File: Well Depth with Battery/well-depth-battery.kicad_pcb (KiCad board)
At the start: 2 copper layers, 40.8 x 48.3 mm, 60 parts, among them J1 Conn_01x02_Female, J2 Conn_01x04_Female, J3 Micro_SD_Card, J4 Conn_01x02_Male, J5 USB_A, J6 Conn_02x05_Odd_Even, Q1 Q_NMOS_GSD, Q2 Q_PMOS_GSD, Q3 Q_PMOS_GSD, U1 LM358, U2 LM358, U3 TL431DBZ, U4 NCP1117-5.0_SOT223, U5 ATSAMD21E17D-M, U6 MCP1793T-3302H/DC, Y1 Crystal_Small

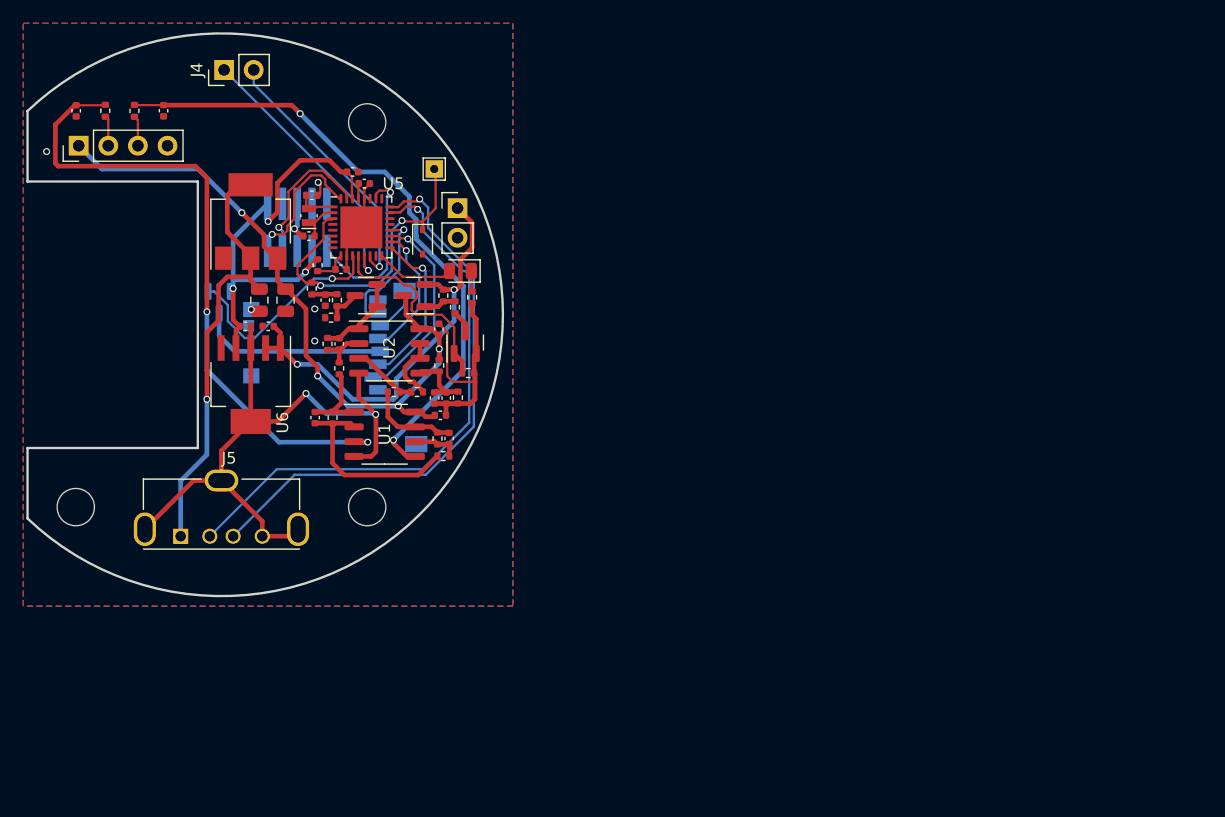
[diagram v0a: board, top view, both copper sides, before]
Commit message: First pass routing for rectangular board
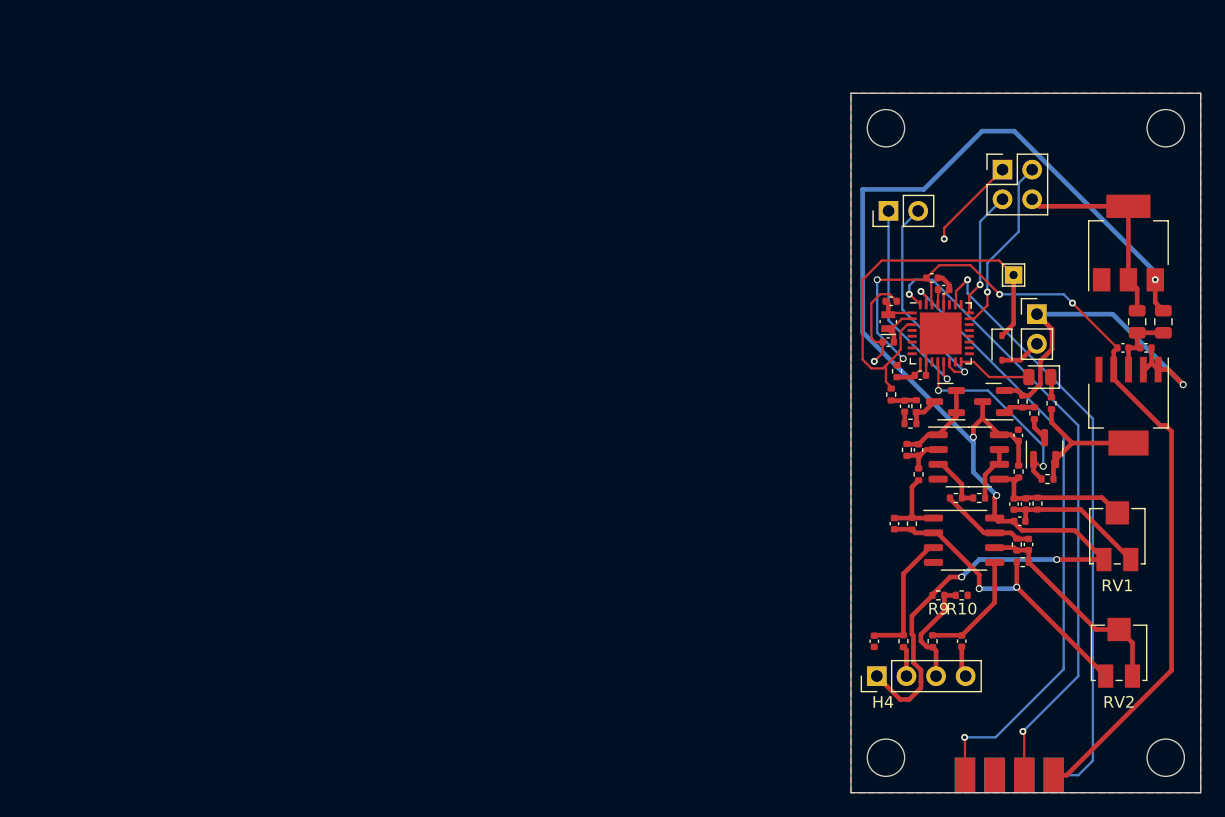
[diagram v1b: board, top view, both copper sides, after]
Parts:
- removed J5: USB_A, Connector_USB:USB_A_Molex_105057_Vertical
- removed Q3: Q_PMOS_GSD, Package_TO_SOT_SMD:SOT-23
- added H4: MountingHole, MountingHole:MountingHole_3.2mm_M3, F.Cu at (143.0, 137.0)
- added R10: 100k, Resistor_SMD:R_0402_1005Metric, F.Cu at (149.5, 123.1)
- added R9: 100k, Resistor_SMD:R_0402_1005Metric, F.Cu at (147.5, 123.1)
- added RV1: 100k, Potentiometer_SMD:Potentiometer_Bourns_3314J_Vertical, F.Cu at (162.8, 118.0)
- added RV2: 1k, Potentiometer_SMD:Potentiometer_Bourns_3314J_Vertical, F.Cu at (163.0, 128.0)
- J3: value Micro_SD_Card -> Conn_02x04_Odd_Even; footprint EWB:MEM2051-00-195-00-A -> EWB:CardEdge_Prog; moved to F.Cu
- J6: value Conn_02x05_Odd_Even -> Conn_01x04; footprint EWB:3221-10-0300-00-TR -> Connector_PinHeader_2.54mm:PinHeader_2x02_P2.54mm_Vertical; moved to F.Cu
- moved C1 82.2 mm to (142.0, 127.0)
- moved C2 82.2 mm to (149.5, 127.0)
- moved R4 82.2 mm to (144.5, 127.0)
- moved R5 82.2 mm to (147.0, 127.0)
- moved J2 82.2 mm to (142.2, 130.0)
- moved H1 76.7 mm to (143.0, 83.0)
- moved C13 75.3 mm to (166.8, 99.6)
- moved C15 75.3 mm to (163.3, 101.8)
- moved C16 75.3 mm to (164.6, 99.6)
- moved U4 75.3 mm to (163.8, 92.8)
- moved C14 75.3 mm to (165.3, 101.8)
- moved U6 75.3 mm to (163.8, 106.8)
- moved H3 71.8 mm to (167.0, 137.0)
- moved J3 70.9 mm to (157.4, 138.5), turned to 180 degrees
- moved H2 68.5 mm to (167.0, 83.0)
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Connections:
- C16 pad 2: Net-(C16-Pad2) -> Net-(J6-Pin_4)
- J3 pad 1: unconnected-(J3-Pad1) -> +3V3
- J3 pad 2: /~{CS} -> /SWDIO
- J3 pad 3: /SDO -> GND
- J3 pad 4: Net-(J3-Pad4) -> /SWCLK
- J3 pad 5: /SCK -> GND
- J3 pad 6: GND -> unconnected-(J3-Pin_6-Pad6)
- J3 pad 7: /SDI -> GND
- J3 pad 8: unconnected-(J3-Pad8) -> /~{SRST}
- J6 pad 1: +3V3 -> GND
- J6 pad 2: /SWDIO -> /USB_D-
- J6 pad 3: GND -> /USB_D+
- J6 pad 4: /SWCLK -> Net-(J6-Pin_4)
- U4 pad 2: Net-(C16-Pad2) -> Net-(J6-Pin_4)
- U5 pad 11: /SD_POW_~{EN} -> unconnected-(U5-PA08-Pad11)
- U5 pad 17: /SDO -> unconnected-(U5-PA16-Pad17)
- U5 pad 18: /SCK -> unconnected-(U5-PA17-Pad18)
- U5 pad 19: /~{CS} -> unconnected-(U5-PA18-Pad19)
- U5 pad 20: /SDI -> unconnected-(U5-PA19-Pad20)
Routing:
- net VDD: track 58.4 -> 119.6 mm, vias 4 -> 5
- net Net-(U1B-+): track 54.7 -> 9.95 mm, vias 2 -> 0
- net Net-(U1A-+): track 55.9 -> 11.3 mm, vias 2 -> 0
- net +3V3: track 37.1 -> 79.0 mm, vias 3 -> 4
- net /SWDIO: track 12.2 -> 54.0 mm, vias 1 -> 2
- net /SWCLK: track 12.6 -> 53.0 mm, vias 1 -> 2
- net /USB_D+: track 48.9 -> 10.9 mm
- net Net-(C16-Pad2): track 37.5 -> 0.00 mm, vias 1 -> 0
- net /~{SRST}: track 14.9 -> 52.2 mm
- net /USB_D-: track 49.3 -> 15.3 mm
- net GND: track 92.1 -> 65.5 mm, vias 8 -> 2
- net /SD_POW_~{EN}: track 18.7 -> 0.00 mm, vias 1 -> 0
- net Net-(J6-Pin_4): track 0.00 -> 17.8 mm
- net /~{CS}: track 17.2 -> 0.00 mm, vias 1 -> 0
- net Net-(J3-Pad4): track 16.3 -> 0.00 mm
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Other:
- board size 40.8 x 48.3 mm -> 30 x 60 mm
- board text removed: "+"
- board text removed: "+9V"
- board text removed: "-"
- board text removed: "GND"
- board text removed: "RX"
- board text removed: "TX"
